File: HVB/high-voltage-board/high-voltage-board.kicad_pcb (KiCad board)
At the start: 2 copper layers, 65 parts, among them J1 Conn_01x23, J10 Conn_01x05, J2 HECS, J3 HV+, J4 HV-, J5 HV+, J6 HV-, J7 Conn_01x02, J9 Bender-LV, Q1 040N03LG, Q2 040N03LG, U2 LTV-817S, U3 LM555xM, U4 LD1117S33TR_SOT223, U5 STM32F413CGUx, U6 MCP2551-I-SN, U7 Vicor_AERO, U8 LTV-817S, U9 TLP184, Y1 Crystal

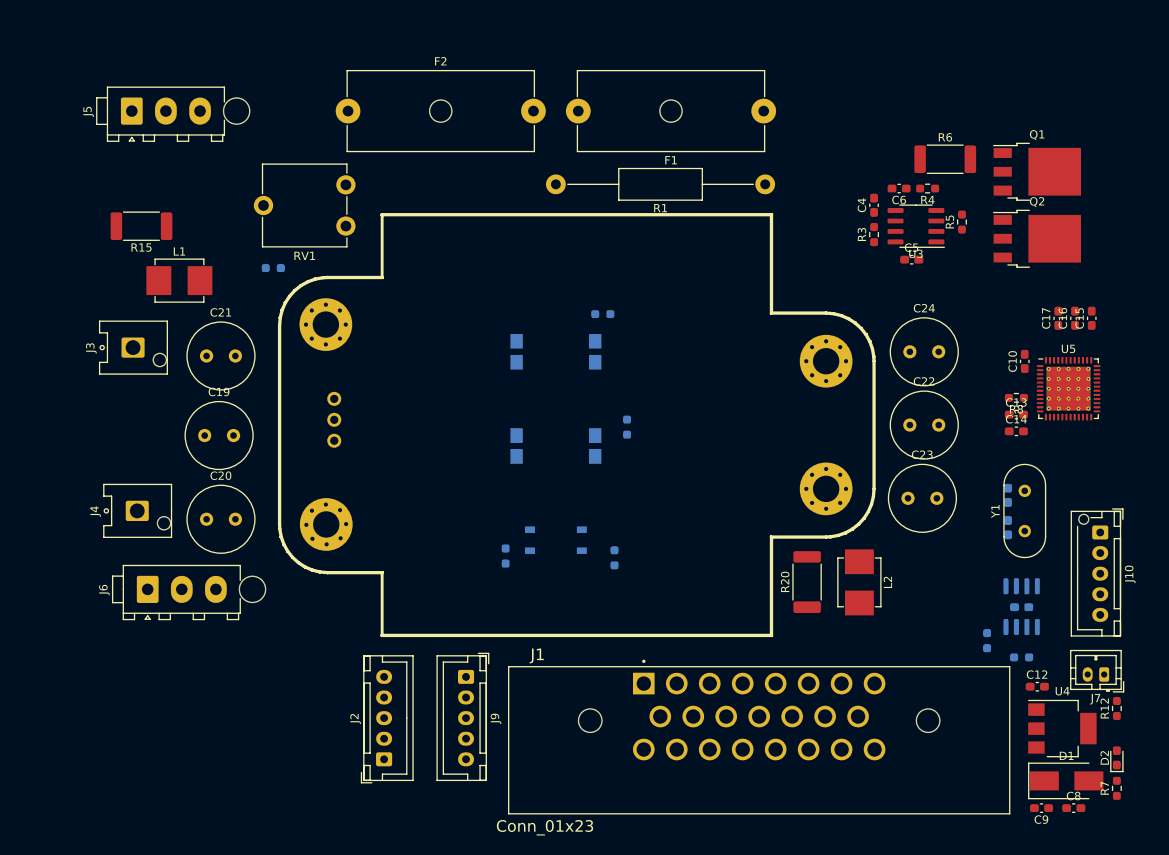
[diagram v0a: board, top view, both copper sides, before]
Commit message: updating trace layout
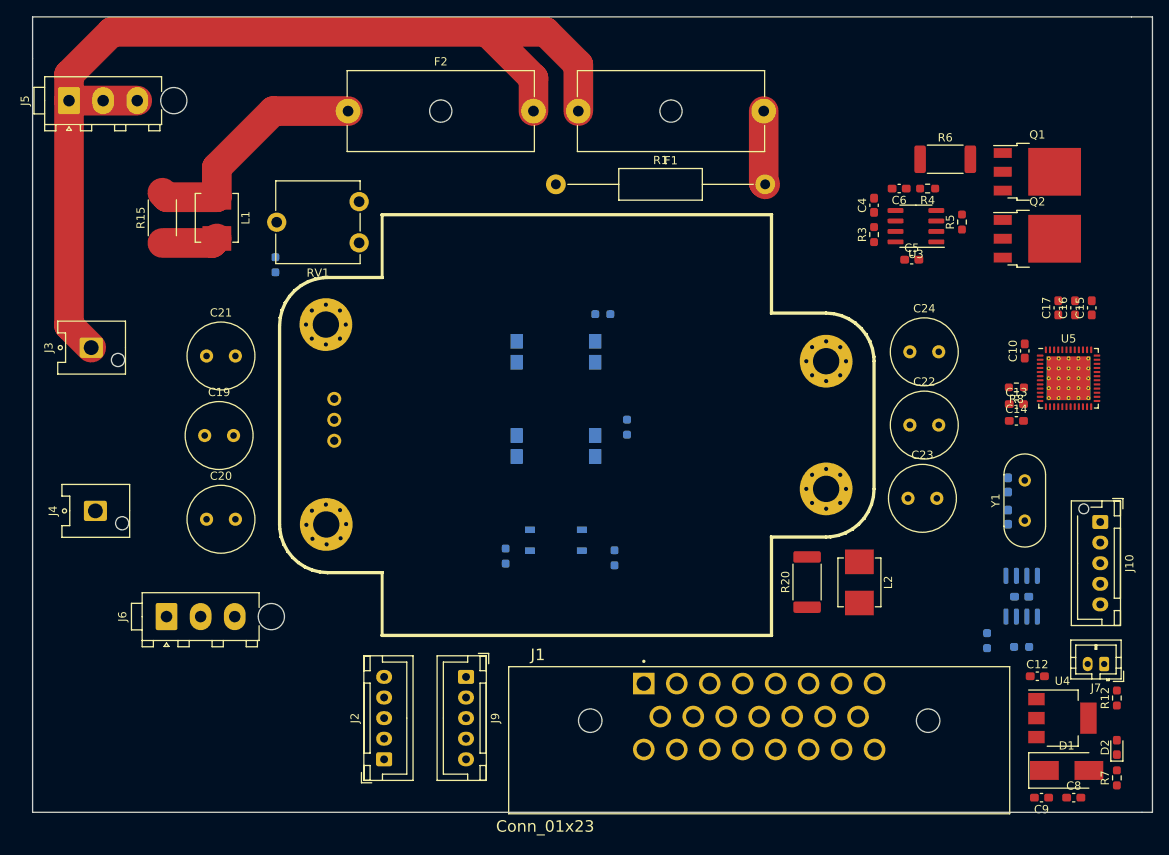
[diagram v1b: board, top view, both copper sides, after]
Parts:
- moved R1 25.4 mm to (88.9, 53.3), turned to 0 degrees
- moved L1 8.87 mm to (47.8, 57.4), turned to -90 degrees
- moved J5 7.73 mm to (29.8, 43.2)
- moved J3 5.08 mm to (32.5, 73.2)
- moved J4 5.08 mm to (33.0, 93.0)
- moved J6 4.02 mm to (41.7, 105.8)
- moved R15 2.73 mm to (41.1, 57.4), turned to 90 degrees
- moved RV1 2.59 mm to (65.0, 55.4)
- moved C15 1.27 mm to (153.9, 68.3)
- moved C16 1.27 mm to (151.9, 68.3)
- moved C17 1.27 mm to (149.9, 68.3)
- moved C8 1.27 mm to (151.7, 127.8)
- moved C9 1.27 mm to (147.8, 127.8)
- moved D1 1.27 mm to (150.9, 124.5)
- moved D2 1.27 mm to (157.0, 121.7)
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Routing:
- net HV+: track 0.00 -> 125.7 mm
- net /vicor/HV+: track 0.00 -> 29.2 mm
- net /TSAL/HV+: track 0.00 -> 8.96 mm
- net Net-(C19-Pad1): track 0.00 -> 6.83 mm
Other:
- board outline added: 135.9 x 96.5 mm

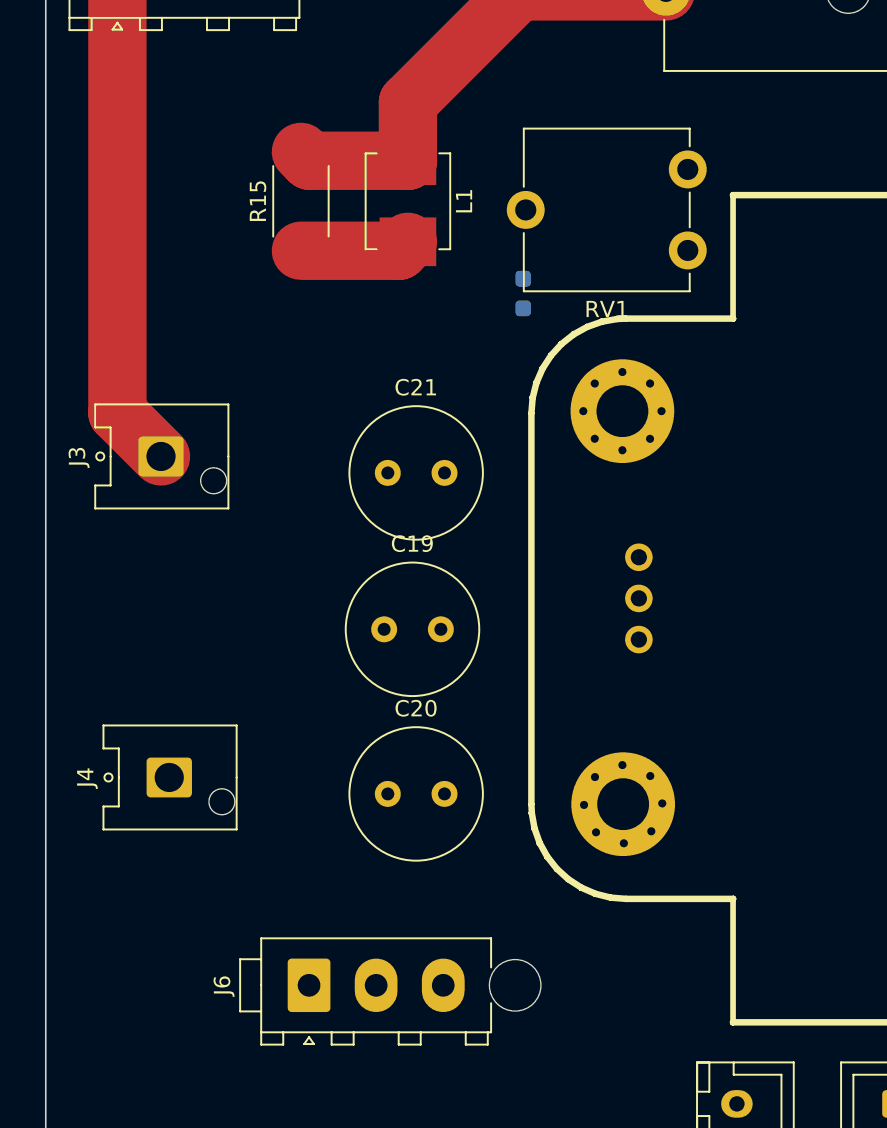
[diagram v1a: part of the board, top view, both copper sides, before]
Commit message: adding traces
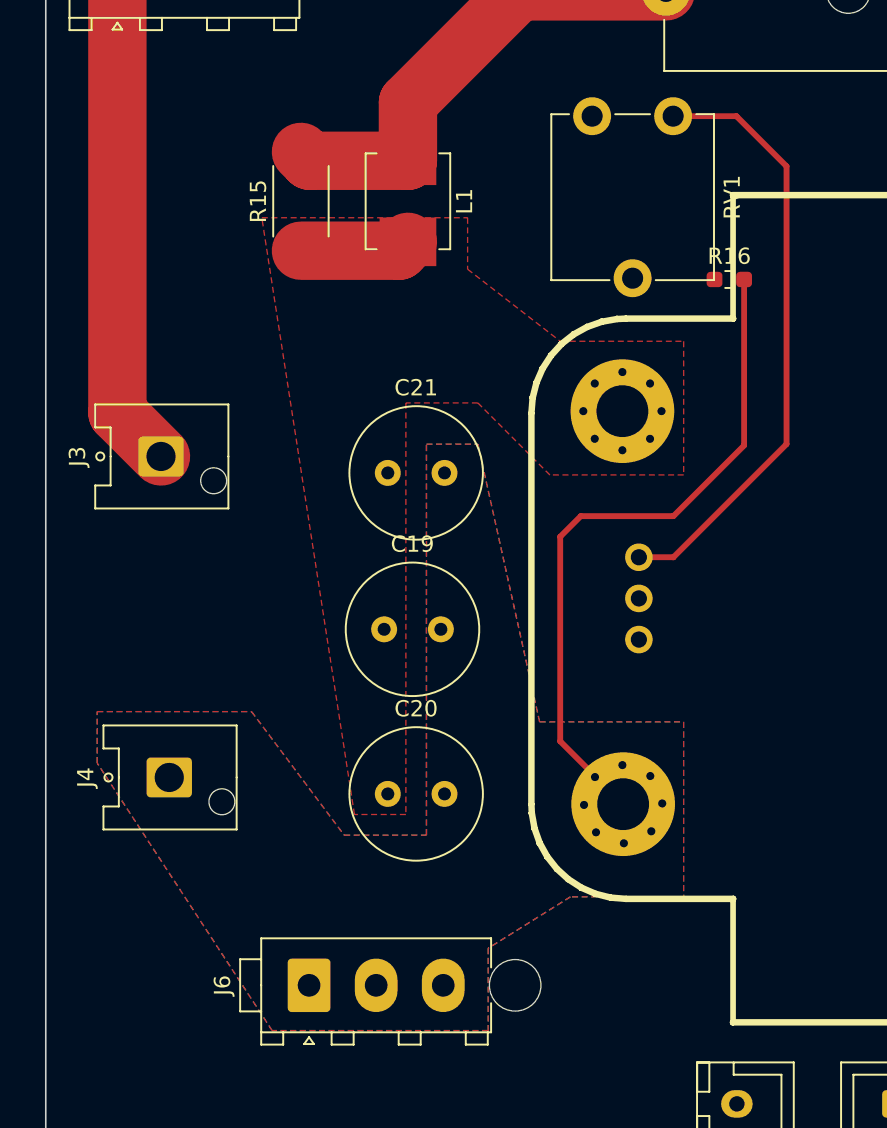
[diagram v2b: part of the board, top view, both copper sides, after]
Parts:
- R16: moved to F.Cu
- moved R16 12.8 mm to (67.6, 62.2), turned to 0 degrees
- moved RV1 6.76 mm to (59.1, 52.1), turned to -90 degrees
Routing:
- net HV-: track 0.00 -> 42.0 mm
- net /vicor/TRIM_HV: track 0.00 -> 37.4 mm
- added copper zone on B.Cu, net HV-
- added copper zone on F.Cu, net HV-
- added copper zone on F.Cu, net Net-(C19-Pad1)
